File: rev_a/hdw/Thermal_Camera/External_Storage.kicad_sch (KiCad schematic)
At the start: 43 parts

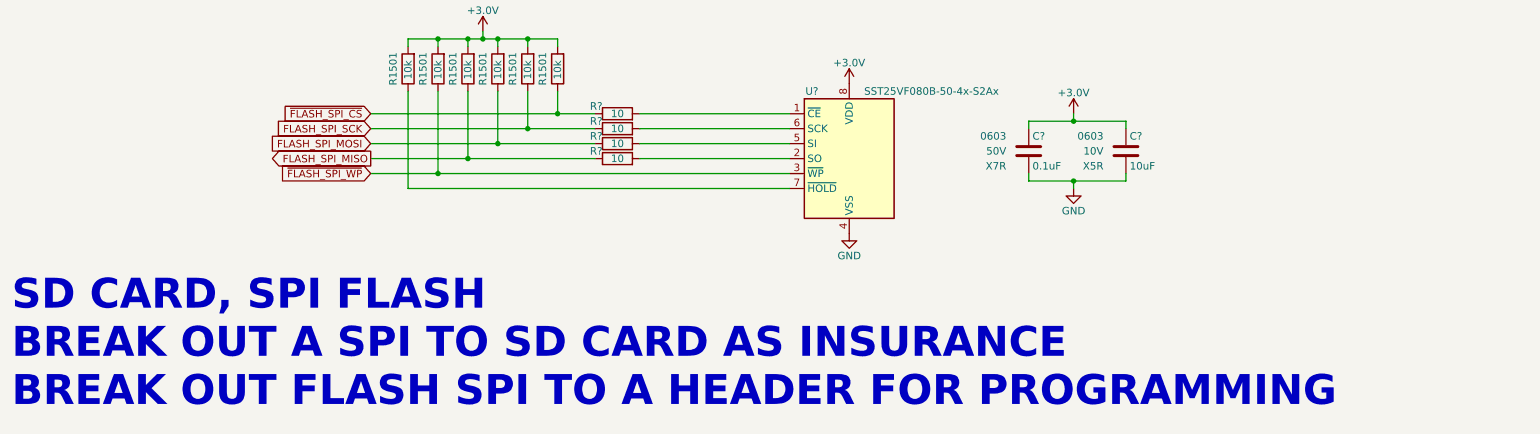
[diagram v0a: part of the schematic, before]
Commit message: added some more USB stuff
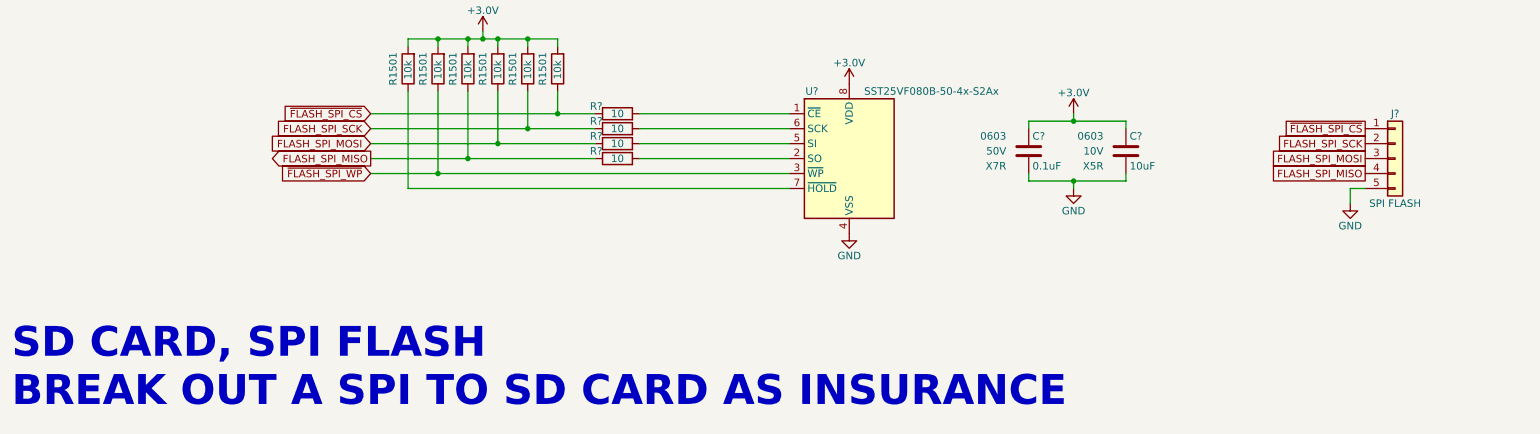
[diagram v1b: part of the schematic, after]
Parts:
- added J?: SPI FLASH, symbol Connector_Generic:Conn_01x05
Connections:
- net FLASH_SPI_MISO: now also J?.4 (Pin_4)
- net FLASH_SPI_MOSI: now also J?.3 (Pin_3)
- net FLASH_SPI_SCK: now also J?.2 (Pin_2)
- net GND: now also J?.5 (Pin_5)
- net ~{FLASH_SPI_CS}: now also J?.1 (Pin_1)
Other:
- note added: "SD CARD, SPI FLASH BREAK OUT A SPI TO SD CARD AS INSURANCE"
- note removed: "SD CARD, SPI FLASH BREAK OUT A SPI TO SD CARD AS INSURANCE BREAK OUT FLASH SPI TO A HEADER FOR PROGRAMMING"
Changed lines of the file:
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@@
     (stroke (width 0) (type default))
   )
+  (wire (pts (xy 237.49 154.94) (xy 237.49 152.4))
+    (stroke (width 0) (type default))
+  )
   (wire (pts (xy 87.63 39.37) (xy 87.63 60.96))
     (stroke (width 0) (type default))
@@
     (stroke (width 0) (type default))
   )
+  (wire (pts (xy 237.49 152.4) (xy 240.03 152.4))
+    (stroke (width 0) (type default))
+  )
   (wire (pts (xy 92.71 91.44) (xy 95.25 91.44))
     (stroke (width 0) (type default))
@@
     (stroke (width 0) (type default))
   )
-  (text "SD CARD, SPI FLASH\nBREAK OUT A SPI TO SD CARD AS INSURANCE\nBREAK OUT FLASH SPI TO A HEADER FOR PROGRAMMING"
+  (text "SD CARD, SPI FLASH\nBREAK OUT A SPI TO SD CARD AS INSURANCE"
     (at 10.16 189.865 0)
     (effects (font (face "Courier New") (size 5.08 5.08) (thickness 1.016) bold (color 194 0 0 1)) (justify left bottom))
@@
     )
   )
+  (global_label "FLASH_SPI_SCK" (shape passive) (at 240.03 144.78 180) (fields_autoplaced)
+    (effects (font (size 1.27 1.27)) (justify right))
+    (property "Intersheetrefs" "${INTERSHEET_REFS}" (at 223.7212 144.78 0)
+      (effects (font (size 1.27 1.27)) (justify right) hide)
+    )
+  )
   (global_label "~{FLASH_SPI_CS}" (shape input) (at 71.12 139.7 180) (fields_autoplaced)
     (effects (font (size 1.27 1.27)) (justify right))
@@
     )
   )
+  (global_label "FLASH_SPI_MOSI" (shape passive) (at 240.03 147.32 180) (fields_autoplaced)
+    (effects (font (size 1.27 1.27)) (justify right))
+    (property "Intersheetrefs" "${INTERSHEET_REFS}" (at 222.8745 147.32 0)
+      (effects (font (size 1.27 1.27)) (justify right) hide)
+    )
+  )
   (global_label "SDHC_SDCK" (shape bidirectional) (at 71.12 53.34 180) (fields_autoplaced)
     (effects (font (size 1.27 1.27)) (justify right))
@@
     )
   )
+  (global_label "~{FLASH_SPI_CS}" (shape passive) (at 240.03 142.24 180) (fields_autoplaced)
+    (effects (font (size 1.27 1.27)) (justify right))
+    (property "Intersheetrefs" "${INTERSHEET_REFS}" (at 224.9912 142.24 0)
+      (effects (font (size 1.27 1.27)) (justify right) hide)
+    )
+  )
   (global_label "SD_PWR_EN" (shape input) (at 92.71 91.44 180) (fields_autoplaced)
     (effects (font (size 1.27 1.27)) (justify right))
@@
     )
   )
+  (global_label "FLASH_SPI_MISO" (shape passive) (at 240.03 149.86 180) (fields_autoplaced)
+    (effects (font (size 1.27 1.27)) (justify right))
+    (property "Intersheetrefs" "${INTERSHEET_REFS}" (at 222.8745 149.86 0)
+      (effects (font (size 1.27 1.27)) (justify right) hide)
+    )
+  )
   (global_label "~{FLASH_SPI_WP}" (shape input) (at 71.12 149.86 180) (fields_autoplaced)
     (effects (font (size 1.27 1.27)) (justify right))
@@
     )
   )
+  (symbol (lib_id "Connector_Generic:Conn_01x05") (at 245.11 147.32 0) (unit 1)
+    (in_bom yes) (on_board yes) (dnp no)
+    (property "Reference" "J?" (at 245.11 139.7 0)
+      (effects (font (size 1.27 1.27)))
+    )
+    (property "Value" "SPI FLASH" (at 245.11 154.94 0)
+      (effects (font (size 1.27 1.27)))
+    )
+    (property "Footprint" "" (at 245.11 147.32 0)
+      (effects (font (size 1.27 1.27)) hide)
+    )
+    (property "Datasheet" "~" (at 245.11 147.32 0)
+      (effects (font (size 1.27 1.27)) hide)
+    )
+    (pin "1")
+    (pin "2")
+    (pin "3")
+    (pin "4")
+    (pin "5")
+    (instances
+      (project "Thermal_Camera"
+        (path "/4bd21e0b-5408-4b93-866e-c82ac5b31fa9/21507370-f247-4205-8e94-91a7207a6f8b"
+          (reference "J?") (unit 1)
+        )
+      )
+    )
+  )
   (symbol (lib_id "power:GND") (at 107.95 104.14 0) (mirror y) (unit 1)
     (in_bom yes) (on_board yes) (dnp no)
@@
         )
       )
+    )
+  )
+  (symbol (lib_id "power:GND") (at 237.49 154.94 0) (unit 1)
+    (in_bom yes) (on_board yes) (dnp no)
+    (property "Reference" "#PWR0190" (at 237.49 161.29 0)
+      (effects (font (size 1.27 1.27)) hide)
+    )
+    (property "Value" "GND" (at 237.49 158.75 0)
+      (effects (font (size 1.27 1.27)))
+    )
+    (property "Footprint" "" (at 237.49 154.94 0)
+      (effects (font (size 1.27 1.27)) hide)
+    )
+    (property "Datasheet" "" (at 237.49 154.94 0)
+      (effects (font (size 1.27 1.27)) hide)
+    )
+    (pin "1")
+    (instances
+      (project "Thermal_Camera"
+        (path "/4bd21e0b-5408-4b93-866e-c82ac5b31fa9/21507370-f247-4205-8e94-91a7207a6f8b"
+          (reference "#PWR0190") (unit 1)
+        )
+      )
